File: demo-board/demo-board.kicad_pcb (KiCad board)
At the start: 2 copper layers, 138 x 32 mm, 22 parts, among them J1 USB_B_Micro, J2 Conn_02x03_Odd_Even, U1 ATtiny85-20SU

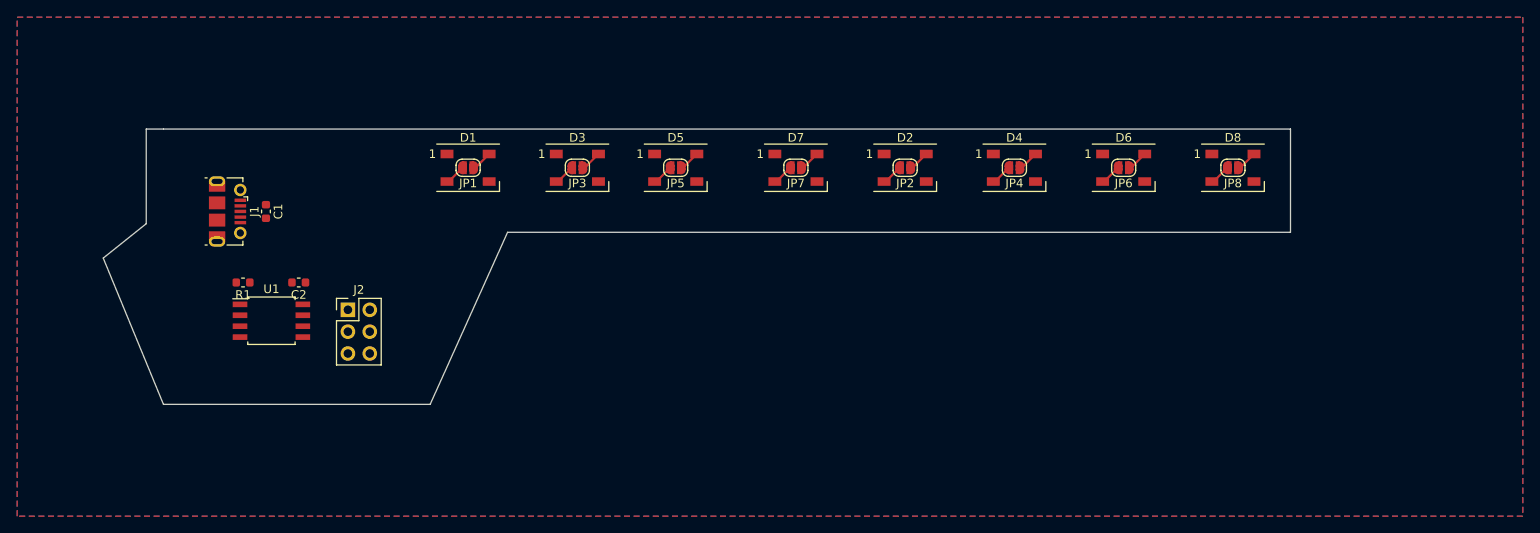
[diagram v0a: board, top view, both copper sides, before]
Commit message: Demo Board updated. Ready for Review
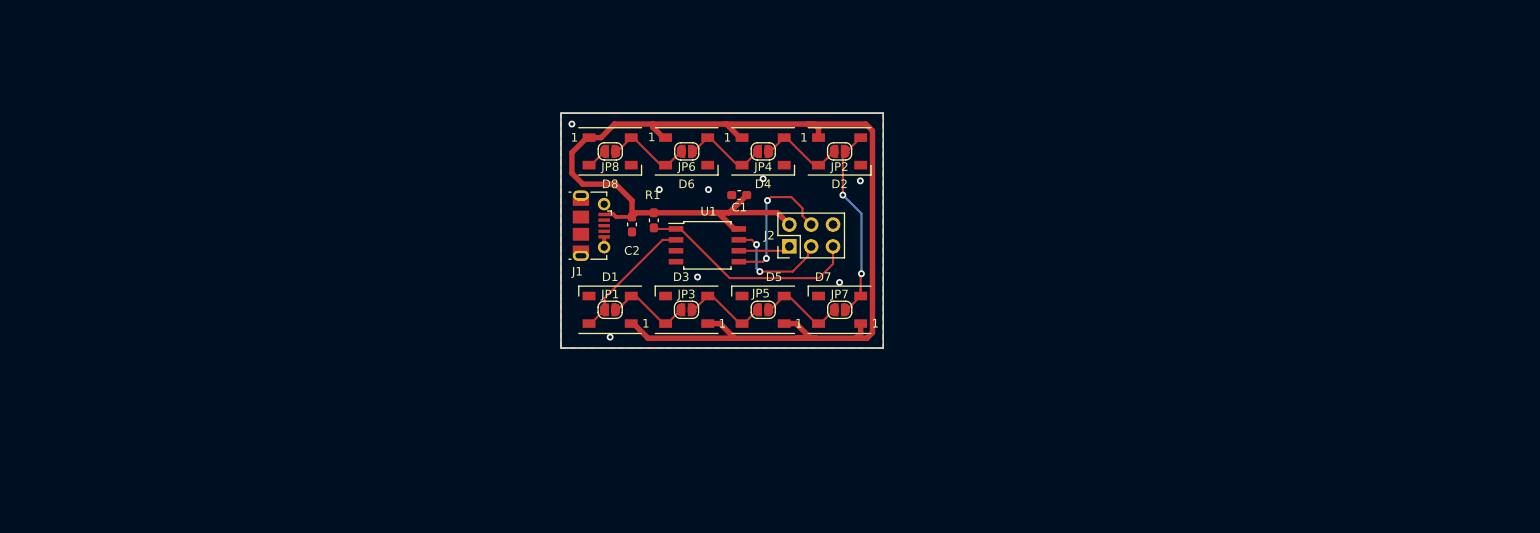
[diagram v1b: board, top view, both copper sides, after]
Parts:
- added G***: LOGO, AERO-footprints:AERO_Logo_15x6mm, B.Cu at (130.2, 80.0)
- C1: value 10u -> 0.1U; footprint Capacitor_SMD:C_0603_1608Metric -> Capacitor_SMD:C_0603_1608Metric_Pad1.05x0.95mm_HandSolder
- C2: value 0.1u -> 10U; footprint Capacitor_SMD:C_0603_1608Metric -> Capacitor_SMD:C_0603_1608Metric_Pad1.05x0.95mm_HandSolder
- R1: value 10k -> 1OK; footprint Resistor_SMD:R_0603_1608Metric -> Resistor_SMD:R_0603_1608Metric_Pad1.05x0.95mm_HandSolder
- moved D8 72.4 mm to (121.9, 61.6)
- moved JP8 72.4 mm to (121.9, 61.6)
- moved C1 55.0 mm to (136.9, 66.7), turned to 180 degrees
- moved J2 51.8 mm to (142.7, 72.6), turned to 90 degrees
- moved U1 51.4 mm to (133.2, 72.5)
- moved D6 50.8 mm to (130.8, 61.6)
- moved JP6 50.8 mm to (130.8, 61.6)
- moved R1 48.3 mm to (127.0, 69.6), turned to 270 degrees
- moved J1 42.3 mm to (119.8, 70.2)
- moved C2 39.3 mm to (124.5, 70.1), turned to 270 degrees
- moved D4 29.3 mm to (139.7, 61.6)
- moved JP4 29.3 mm to (139.7, 61.6)
- moved D1 23.3 mm to (121.9, 80.0), turned to 180 degrees
- moved JP1 23.3 mm to (121.9, 80.0), turned to 0 degrees
- moved D3 20.8 mm to (130.8, 80.0), turned to 180 degrees
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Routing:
- net +5V: track 0.00 -> 153.6 mm
- net /RST: track 0.00 -> 26.0 mm
- net Net-(D2-Pad4): track 4.93 -> 23.6 mm, vias 0 -> 2
- net /MOSI: track 0.00 -> 17.2 mm, vias 0 -> 2
- net Net-(D1-Pad4): track 2.46 -> 15.9 mm
- net /SCK: track 0.00 -> 13.2 mm, vias 0 -> 2
- net /MISO: track 0.00 -> 6.09 mm
- net Net-(D3-Pad2): track 4.93 -> 10.3 mm
- net Net-(D6-Pad2): track 4.93 -> 10.2 mm
- net Net-(D4-Pad2): track 4.93 -> 10.2 mm
- net Net-(D5-Pad2): track 4.93 -> 10.2 mm
- net Net-(D1-Pad2): track 4.93 -> 10.2 mm
- net Net-(D2-Pad2): track 4.93 -> 10.2 mm
- net GND: track 0.00 -> 1.22 mm, vias 0 -> 8
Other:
- board size 138 x 32 mm -> 37.5 x 27.3 mm
- net class Default: clearance 0.254 -> 0.2; trace_width 0.254 -> 0.25
- net class Power: clearance 0.3048 -> 0.254
- rule trace_clearance: 0.254 -> 0.2
- board text added: "George Spearing October 2019 Demo RGB"
